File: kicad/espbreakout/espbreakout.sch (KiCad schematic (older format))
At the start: 21 parts, among them J1 TEMPERATURE, J2 POWER, J3 CURRENT, J4 LED DATA, J5 RELAY, J6 Conn_01x19, J7 Conn_01x19, J8 I2C, J9 SERIAL

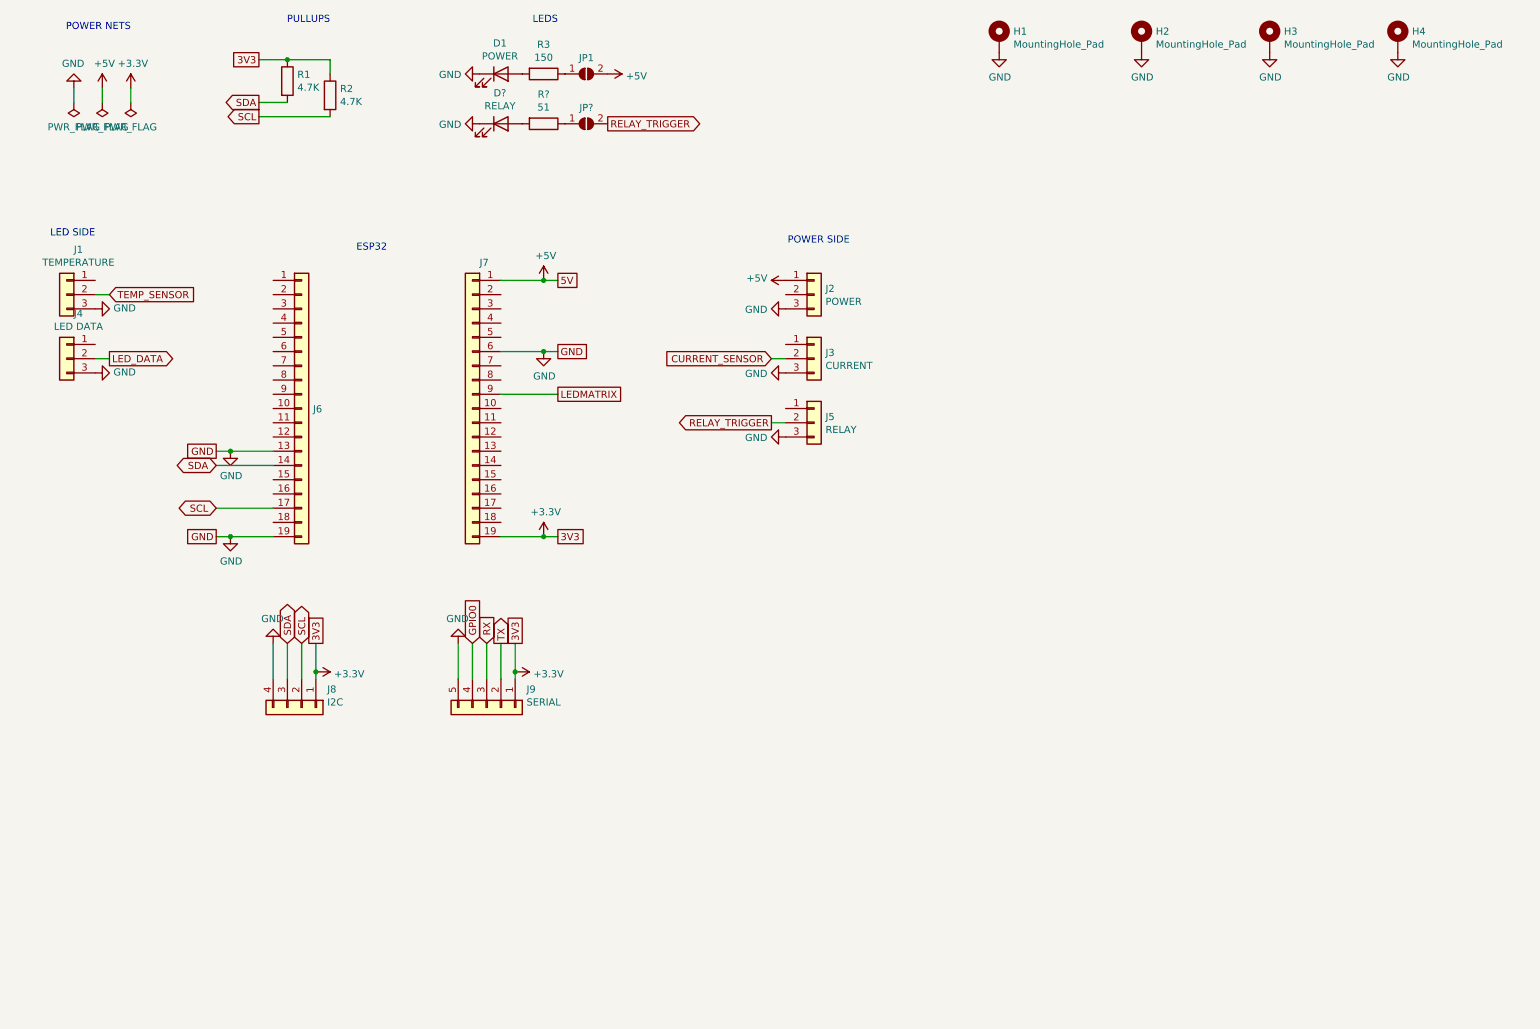
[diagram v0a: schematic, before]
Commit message: esp breakout
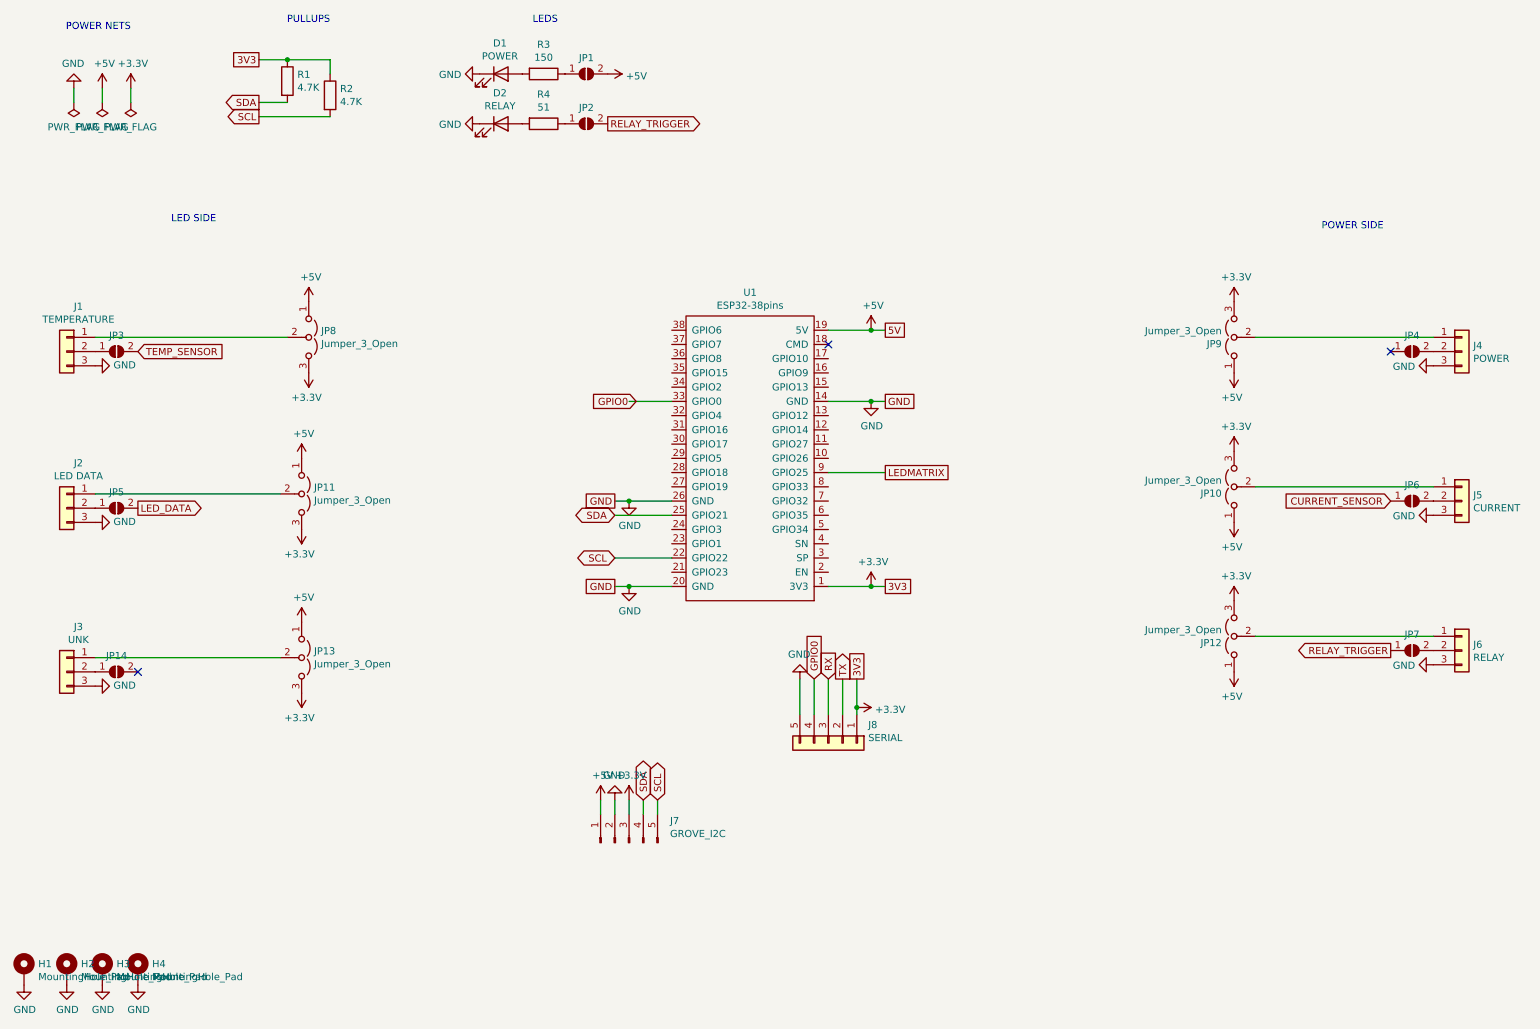
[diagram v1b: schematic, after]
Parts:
- removed J6, J7: Conn_01x19, Pin_Headers:Pin_Header_Straight_1x19_Pitch2.54mm, symbol Connector_Generic:Conn_01x19
- removed J8: I2C, Pin_Headers:Pin_Header_Straight_1x04_Pitch2.54mm, symbol Connector_Generic:Conn_01x04
- added J3: UNK, Connectors_Phoenix:PhoenixContact_MCV-G_03x3.81mm_Vertical, symbol Connector_Generic:Conn_01x03
- added J7: GROVE_I2C, Connectors_JST:JST_PH_S5B-PH-K_05x2.00mm_Angled, symbol Connector:Conn_01x05_Male
- added JP10, JP11, JP12, JP13, JP8, JP9: Jumper_3_Open, Jumper:SolderJumper-3_P1.3mm_Open_Pad1.0x1.5mm, symbol Jumper:Jumper_3_Open
- added JP14, JP3, JP5: SolderJumper_2_Open, Jumper:SolderJumper-2_P1.3mm_Open_TrianglePad1.0x1.5mm, symbol Jumper:SolderJumper_2_Open
- added JP4, JP6, JP7: D, Jumper:SolderJumper-2_P1.3mm_Open_TrianglePad1.0x1.5mm, symbol Jumper:SolderJumper_2_Open
- added U1: ESP32-38pins, drz-lib:esp32 38pin azdelivery, symbol drz-symbols:ESP32-38pins
- J1: footprint Pin_Headers:Pin_Header_Straight_1x03_Pitch2.54mm -> Connectors_Phoenix:PhoenixContact_MCV-G_03x3.81mm_Vertical
- J2: renamed from J4; footprint Pin_Headers:Pin_Header_Straight_1x03_Pitch2.54mm -> Connectors_Phoenix:PhoenixContact_MCV-G_03x3.81mm_Vertical
- J4: renamed from J2; footprint Pin_Headers:Pin_Header_Straight_1x03_Pitch2.54mm -> Connectors_Phoenix:PhoenixContact_MCV-G_03x3.81mm_Vertical
- J5: renamed from J3; footprint Pin_Headers:Pin_Header_Straight_1x03_Pitch2.54mm -> Connectors_Phoenix:PhoenixContact_MCV-G_03x3.81mm_Vertical
- J6: renamed from J5; footprint Pin_Headers:Pin_Header_Straight_1x03_Pitch2.54mm -> Connectors_Phoenix:PhoenixContact_MCV-G_03x3.81mm_Vertical
- gave numbers to parts that had none: 3
- renumbered J9 to J8
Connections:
- net +3V3: now also J7.3 (Pin_3), JP10.3 (B), JP11.3 (B), JP12.3 (B), JP13.3 (B), JP8.3 (B), JP9.3 (B), U1.1 (3V3)
- net +5V: now also J7.1 (Pin_1), JP10.1 (A), JP11.1 (A), JP12.1 (A), JP13.1 (A), JP8.1 (A), JP9.1 (A), U1.19 (5V); no longer J4.1 (Pin_1)
- net CURRENT_SENSOR: now also JP6.1 (A); no longer J5.2 (Pin_2)
- net GND: now also J3.3 (Pin_3), J7.2 (Pin_2), U1.14 (GND), U1.20 (GND), U1.26 (GND)
- net GPIO0: now also U1.33 (GPIO0)
- net LEDMATRIX: now also U1.9 (GPIO25)
- net LED_DATA: now also JP5.2 (B); no longer J2.2 (Pin_2)
- net RELAY_TRIGGER: now also JP7.1 (A); no longer J6.2 (Pin_2)
- net SCL: now also J7.5 (Pin_5), U1.22 (GPIO22)
- net SDA: now also J7.4 (Pin_4), U1.25 (GPIO21)
- net TEMP_SENSOR: now also JP3.2 (B); no longer J1.2 (Pin_2)
- net at J4.2 (Pin_2): now also JP4.2 (B)
- net at J5.1 (Pin_1): now also JP10.2 (C)
- net at J6.1 (Pin_1): now also JP12.2 (C)
- net at J2.1 (Pin_1): now also JP11.2 (C)
- net at J1.1 (Pin_1): now also JP8.2 (C)
- new net: J4.1 (Pin_1), JP9.2 (C)
- new net: J5.2 (Pin_2), JP6.2 (B)
- new net: J6.2 (Pin_2), JP7.2 (B)
- new net: J2.2 (Pin_2), JP5.1 (A)
- new net: J1.2 (Pin_2), JP3.1 (A)
- new net: J3.1 (Pin_1), JP13.2 (C)
- new net: J3.2 (Pin_2), JP14.1 (A)
- no-connect marks 0 -> 3
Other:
- note removed: "ESP32"
- moved on the sheet: H1, H2, H3, H4, J1, J2, J4, J5, J6, J8
